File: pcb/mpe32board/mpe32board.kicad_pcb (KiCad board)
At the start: 4 copper layers, 107 x 87 mm, 204 parts, among them J1 Conn_ST_STDC14, J10 Conn_01x04, J11 Conn_01x04, J12 Conn_01x04, J13 Conn_01x04, J14 Conn_01x04, J15 Conn_01x04, J16 Conn_01x04, J17 Conn_01x04, J18 Conn_01x04, J19 Conn_01x04, J2 USB_C_Receptacle_USB2.0_16P, J20 Conn_01x04, J21 Conn_01x04, J22 Conn_01x04, J23 Conn_01x04, J24 Conn_01x04, J25 Conn_01x04, J26 Conn_01x04, J27 Conn_01x04, J28 Conn_01x04, J29 Conn_01x04, J3 Conn_01x01_Socket, J30 Conn_01x04, J31 Conn_01x04, J32 Conn_01x04, J33 Conn_01x04, J34 Conn_01x04, J35 Conn_01x04, J36 Conn_01x04, J37 Conn_01x04, J38 Conn_01x04, J39 Conn_01x04, J4 Conn_01x04, J40 Conn_01x04, J41 Conn_01x04, J42 Conn_01x04, J43 Conn_01x04, J44 Micro_SD_Card, J45 Conn_01x04_Socket, J46 Conn_02x10_Counter_Clockwise, J47 AudioJack3_Ground, J5 Conn_01x04, J6 Conn_01x04, J7 Conn_01x04, J8 Conn_01x04, J9 Conn_01x04, SW1 SW_Push, SW2 SW_Push, SW3 SW_Push, SW4 SW_Push, SW5 SW_Push, SW6 SW_Push, U1 TAC5212IRGER, U10 W9812G6KH-75, U2 USBLC6-2P6, U3 AMS1117-3.3, U4 TCA9548ARGER, U5 TCA9548ARGER, U6 TCA9548ARGER, U7 TCA9548ARGER, U8 TCA9548ARGER, U9 STM32H743IITx

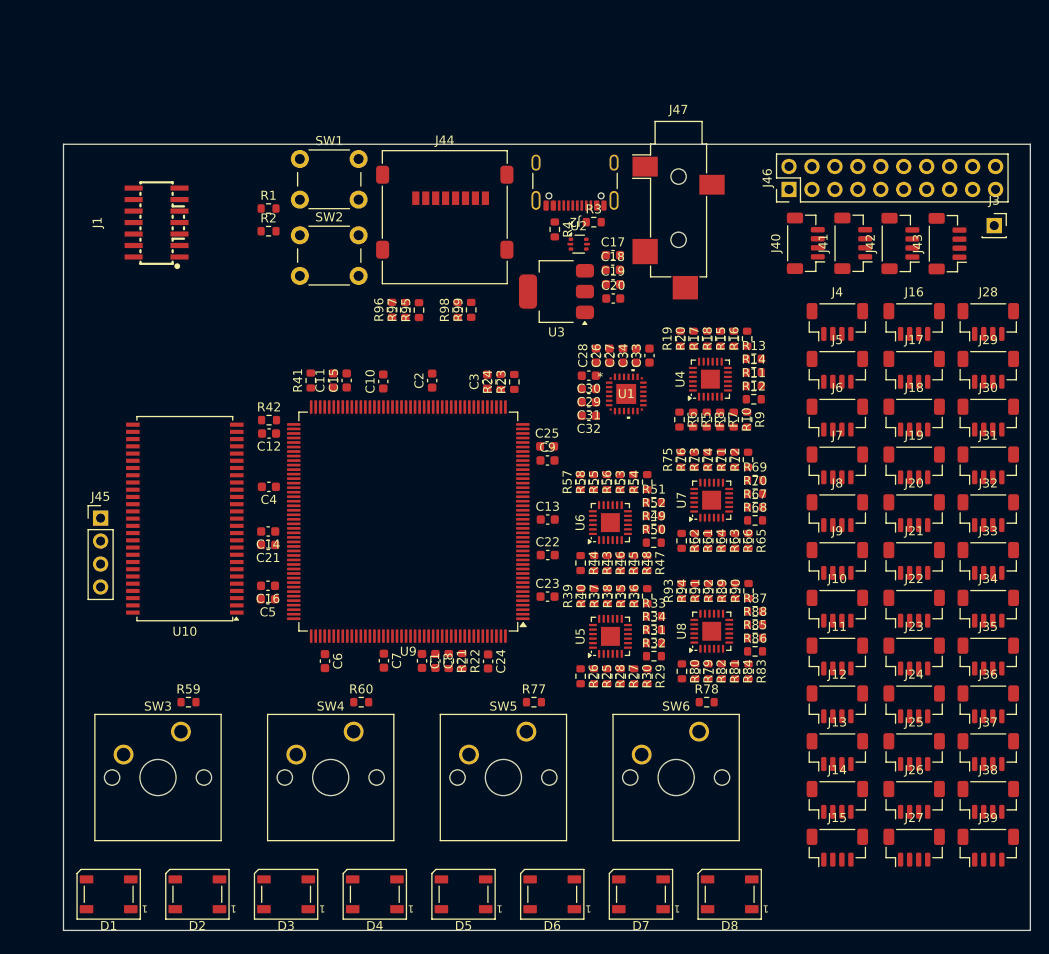
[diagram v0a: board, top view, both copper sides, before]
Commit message: board layout stuff
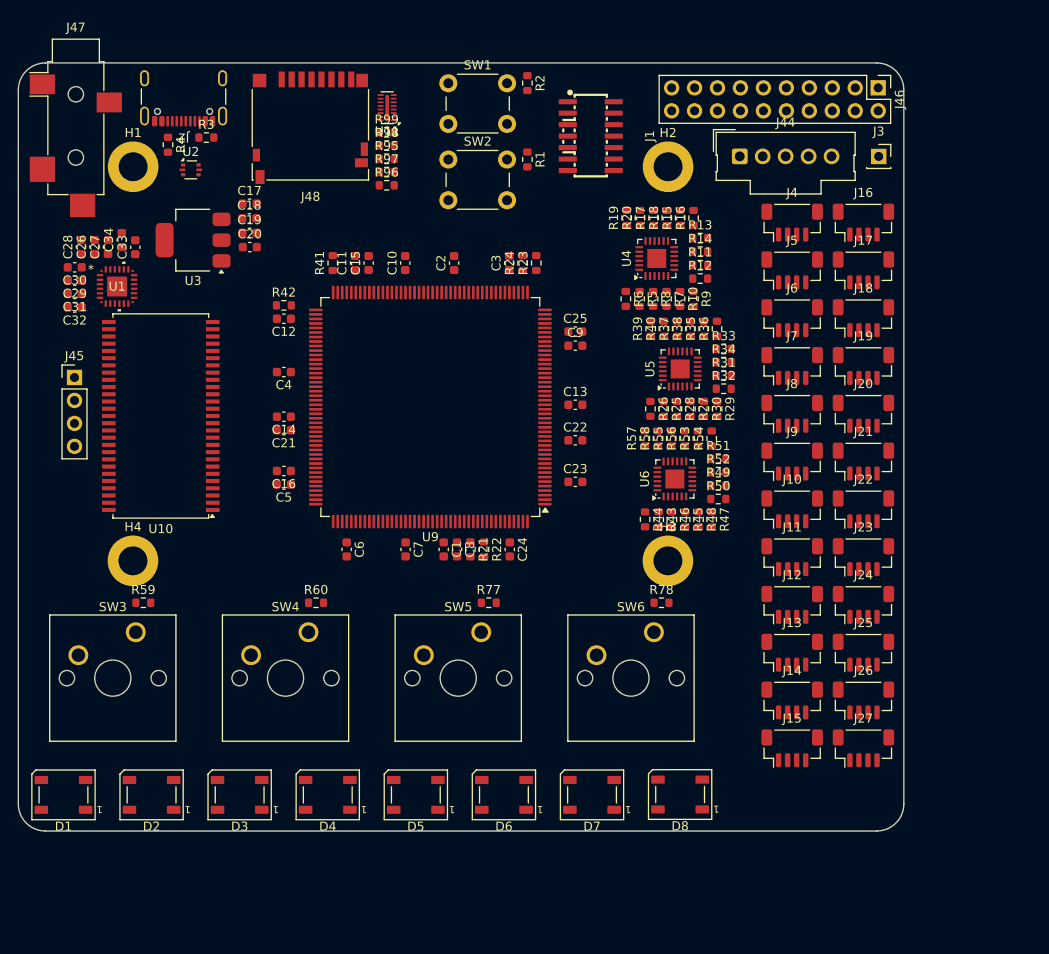
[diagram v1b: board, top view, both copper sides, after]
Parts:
- removed J28, J29, J30, J31, J32, J33, J34, J35, J36, J37, J38, J39, J40, J41, J42, J43: Conn_01x04, Connector_JST:JST_SH_BM04B-SRSS-TB_1x04-1MP_P1.00mm_Vertical
- removed R61, R62, R63, R64, R65, R66, R67, R68, R69, R70, R71, R72, R73, R74, R75, R76, R79, R80, R81, R82, R83, R84, R85, R86, R87, R88, R89, R90, R91, R92, R93, R94: 2.2kΩ, Resistor_SMD:R_0603_1608Metric
- removed U7, U8: TCA9548ARGER, Package_DFN_QFN:Texas_RGE0024C_VQFN-24-1EP_4x4mm_P0.5mm_EP2.1x2.1mm
- added H1: MountingHole_Pad, MountingHole:MountingHole_3.2mm_M3_DIN965_Pad, F.Cu at (72.7, 91.5)
- added H2: MountingHole_Pad, MountingHole:MountingHole_3.2mm_M3_DIN965_Pad, F.Cu at (131.9, 91.5)
- added H3: MountingHole_Pad, MountingHole:MountingHole_3.2mm_M3_DIN965_Pad, F.Cu at (131.9, 135.1)
- added H4: MountingHole_Pad, MountingHole:MountingHole_3.2mm_M3_DIN965_Pad, F.Cu at (72.7, 135.1)
- added J48: Micro_SD_Card_Det_Hirose_DM3AT, Connector_Card:microSD_HC_Hirose_DM3D-SF, F.Cu at (92.3, 87.2)
- added U11: IP4252CZ16, Package_SON:Nexperia_HUSON-16_USON-16-1EP_1.35x3.3mm_P0.4mm_EP0.4x2.8mm, F.Cu at (100.8, 85.0)
- J44: value Micro_SD_Card -> Conn_01x05; footprint Connector_Card:microSD_HC_Molex_47219-2001 -> Connector_Molex:Molex_SL_171971-0005_1x05_P2.54mm_Vertical
- moved J47 67.3 mm to (66.4, 86.0)
- moved C34 58.4 mm to (71.5, 99.6)
- moved C26 58.2 mm to (68.4, 100.4)
- moved C27 58.2 mm to (69.9, 100.4)
- moved C28 58.2 mm to (66.9, 100.4)
- moved C33 58.1 mm to (73.0, 100.4)
- moved C29 58.1 mm to (66.3, 104.1)
- moved C30 58.1 mm to (66.2, 102.6)
- moved C31 58.1 mm to (66.3, 105.6)
- moved C32 58.1 mm to (66.3, 107.1)
- moved U1 57.6 mm to (70.9, 104.7)
- moved J1 49.0 mm to (123.3, 88.1), turned to -90 degrees
- moved J2 44.3 mm to (78.3, 82.8)
- moved R3 43.9 mm to (80.8, 88.3)
- moved R4 43.8 mm to (76.6, 89.1)
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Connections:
- J44 pad 1: SDMMC1_D2 -> +3V3
- J44 pad 2: SDMMC1_D3 -> I2C2_SCL
- J44 pad 3: SDMMC1_CMD -> I2C2_SDA
- J44 pad 4: +3V3 -> RESET_0
- J44 pad 5: SDMMC1_CK -> GND
- U9 pad 134: unconnected-(U9-PI3-Pad134) -> BTN4_INTERNAL
- U9 pad 173: unconnected-(U9-PI4-Pad173) -> BTN3_INTERNAL
- U9 pad 174: unconnected-(U9-PI5-Pad174) -> BTN2_INTERNAL
- U9 pad 175: unconnected-(U9-PI6-Pad175) -> BTN1_INTERNAL
- U9 pad 41: unconnected-(U9-PA1-Pad41) -> SDCARD_DET
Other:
- board size 107 x 87 mm -> 98 x 85 mm
